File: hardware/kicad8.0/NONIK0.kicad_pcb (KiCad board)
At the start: 2 copper layers, 55 x 22 mm, 26 parts, among them J1 AVR-UPDI-3, J2 Qwiic/Stemma QT, J3 Test Pads, J4 Test Pads, Q1 S8050, SW1 SW_SPST, SW2 SW_Push, SW3 SW_Push, U1 LED_HCMS-2915, U2 ATtiny1604-SS, U3 AP3602A

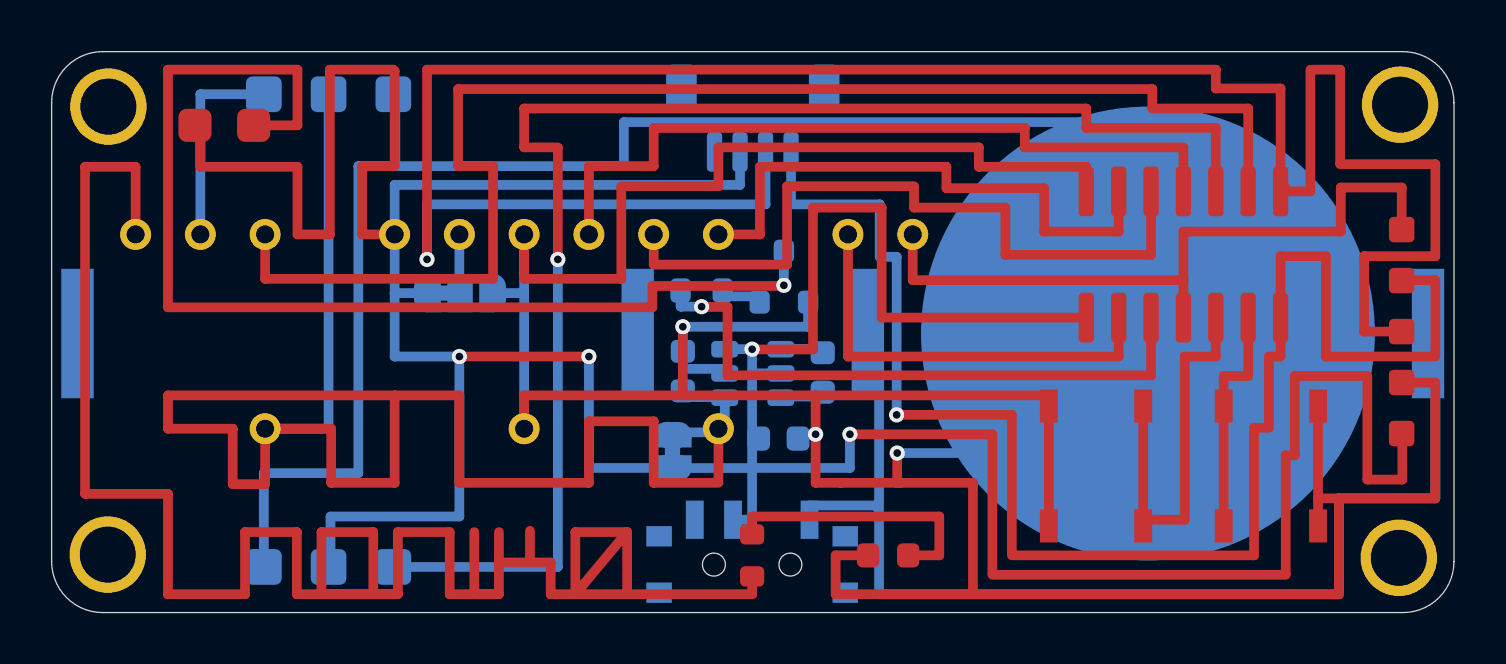
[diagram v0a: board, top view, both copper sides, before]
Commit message: fit and finish
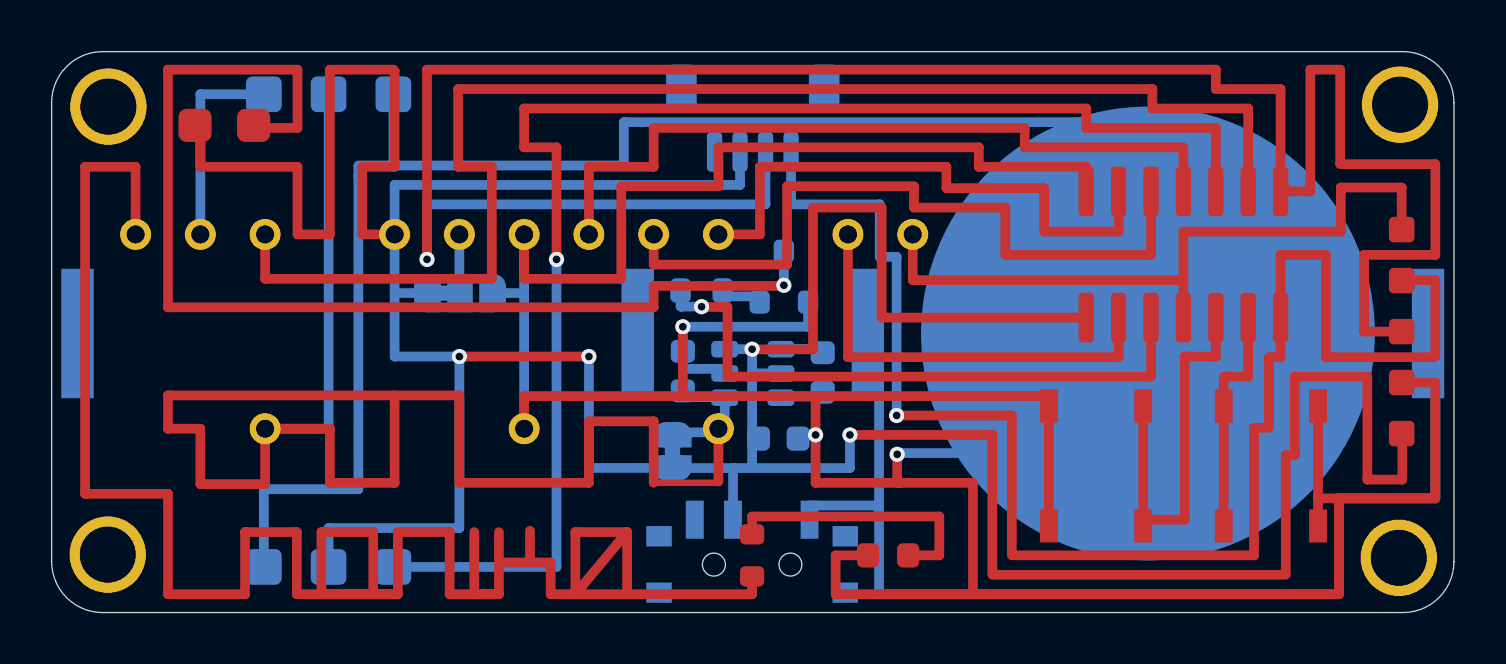
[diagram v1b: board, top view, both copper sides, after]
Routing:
- net VCC: track 162.3 -> 161.3 mm

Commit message: pcb fixes, in progress
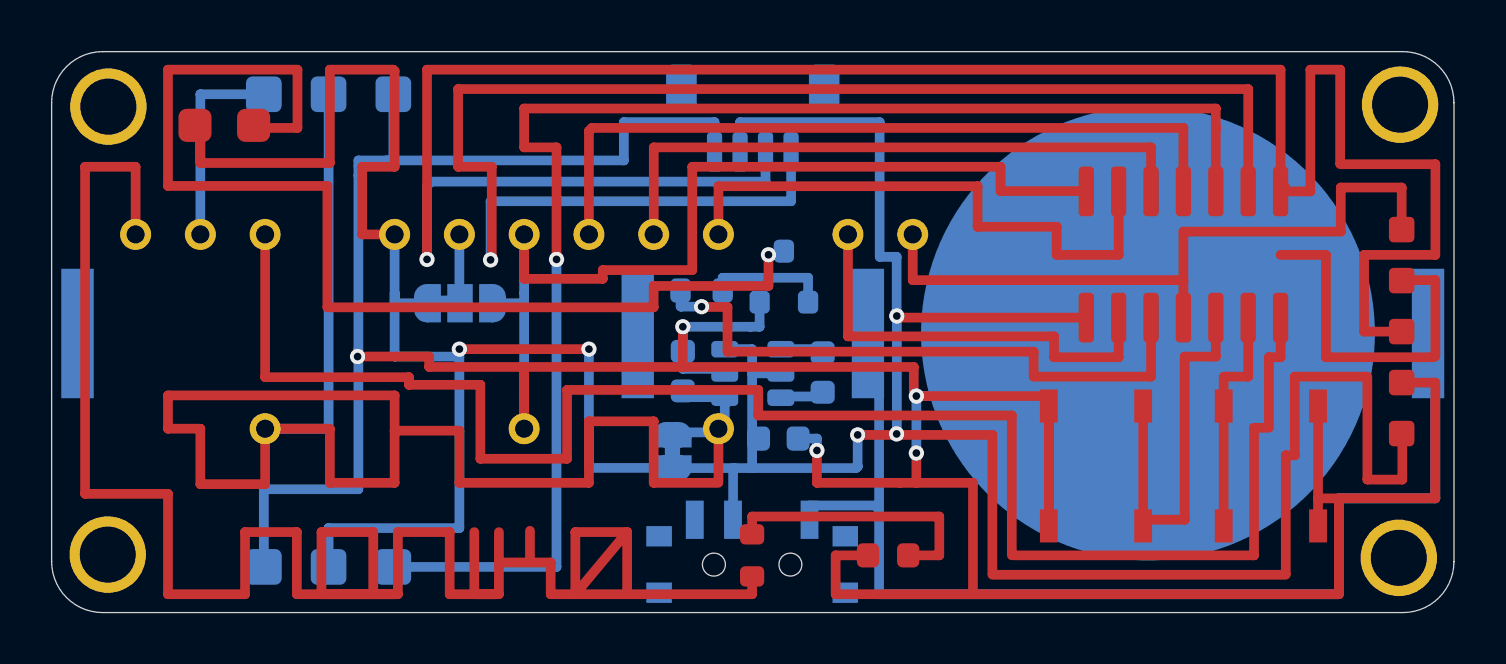
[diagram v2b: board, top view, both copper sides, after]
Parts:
- moved JP2 0.40 mm to (58.9, 27.5)
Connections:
- U2 pad 7: SCL -> RESET
- U2 pad 9: RESET -> SCL
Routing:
- net VCC: track 161.3 -> 143.7 mm, vias 4 -> 5
- net RESET: track 54.4 -> 67.1 mm
- net SCL: track 61.5 -> 73.5 mm
- net GND: track 230.7 -> 221.9 mm, vias 3 -> 5
- net CE: track 28.9 -> 24.6 mm
- net Net-(Q1-B): track 1.45 -> 4.82 mm
- net Vled: track 73.0 -> 71.7 mm
- net Net-(BZ1--): track 44.8 -> 44.1 mm
